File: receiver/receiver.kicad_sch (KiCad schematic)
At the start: 0 parts

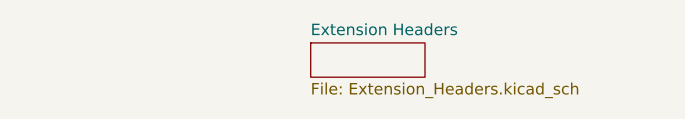
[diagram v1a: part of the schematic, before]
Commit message: First draft of new board
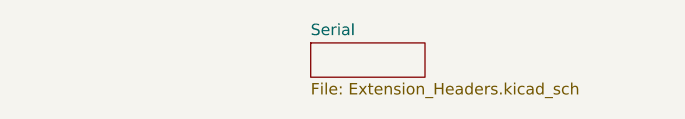
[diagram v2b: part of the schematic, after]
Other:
- sheet Extension Headers renamed Serial
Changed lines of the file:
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@@
 			(project "receiver"
 				(path "/778027c0-3525-441e-8e71-ce93a37417d3"
-					(page "4")
+					(page "5")
 				)
 			)
@@
 			(project "receiver"
 				(path "/778027c0-3525-441e-8e71-ce93a37417d3"
-					(page "3")
+					(page "4")
 				)
 			)
@@
 			(project "receiver"
 				(path "/778027c0-3525-441e-8e71-ce93a37417d3"
-					(page "2")
+					(page "3")
 				)
 			)
@@
 			(color 0 0 0 0.0000)
 		)
-		(property "Sheetname" "Extension Headers"
+		(property "Sheetname" "Serial"
 			(at 228.6 24.6884 0)
 			(effects
@@
 			(project "receiver"
 				(path "/778027c0-3525-441e-8e71-ce93a37417d3"
-					(page "5")
+					(page "2")
 				)
 			)
